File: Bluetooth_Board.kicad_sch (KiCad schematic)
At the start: 67 parts, among them IC1 STM32WB55CGU6, J1 USART1_Headers, J10 Debug_Pins, J12 Power_Selector_Jumper, J13 General_Pin_Header, J14 JST_XH_2.54_Plug, J15 LPUART1_Headers, J16 SPI1_Headers, J19 3V_Selection_Header, J2 SMA PCB END LAUNCH JACK ROUND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, J3 User Button Jumper, J4 Coin Battery Jumper, J5 USB_B_Micro, J6 I2C1_Headers, J7 General_Pin_Header, J8 BOOT0_Jumper, Q1 MOSFET_SI2333DDS-T1-BE3, U3 USBLC6-2SC6, Y4 ABM3B-32.000MHZ-8-R30-B1U-T

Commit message: Update
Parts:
- removed BH1: Battery_Holder_1060TR, Personal_Project:Battery_Holder_1060TR, symbol Personal_Projects:Battery_Holder_1060TR
- removed C12: 0p8 GRM1555C1HR80BA01D, Capacitor_SMD:C_0402_1005Metric_Pad0.74x0.62mm_HandSolder, symbol Device:C
- removed C19: 10n, Capacitor_SMD:C_0805_2012Metric, symbol Device:C
- removed C2, C28, C31, C32: 4u7, Capacitor_SMD:C_0805_2012Metric, symbol Device:C
- removed C20, C21, C22, C27, C29, C30, C33, C34: 100n, Capacitor_SMD:C_0805_2012Metric, symbol Device:C
- removed C24, C25, C35: 1u, Capacitor_SMD:C_0805_2012Metric, symbol Device:C
- removed C36, C9: 1uF, Capacitor_SMD:C_0805_2012Metric, symbol Device:C
- removed C7: 0p3 GRM1555C1HR30WA01D, Capacitor_SMD:C_0402_1005Metric_Pad0.74x0.62mm_HandSolder, symbol Device:C
- removed D1: BZX84C4V3LT1G, Package_TO_SOT_SMD:SOT-23, symbol Diode:BZX84Cxx
- removed D2: BZX84C6V2LT1G, Package_TO_SOT_SMD:SOT-23, symbol Diode:BZX84Cxx
- removed FB1: BLM21PG601SN1D_0805, Capacitor_SMD:C_0805_2012Metric, symbol Device:FerriteBead
- removed FLT1: DLF162500LT-5028A1, Personal_Project:DLF162500LT-5028A1, symbol Personal_Projects:DLF162500LT-5028A1
- removed H1, H2, H3, H4: MountingHole_Pad, MountingHole:MountingHole_3.2mm_M3_Pad, symbol Mechanical:MountingHole_Pad
- removed IC1: STM32WB55CGU6, Personal_Project:STM32WB55CGU6_QFN50P700X700X60-49N-D, symbol Personal_Projects:STM32WB55CGU6
- removed J1: USART1_Headers, Connector_PinHeader_2.54mm:PinHeader_2x03_P2.54mm_Horizontal, symbol Connector_Generic:Conn_02x03_Odd_Even
- removed J10: Debug_Pins, Connector_PinHeader_2.54mm:PinHeader_2x04_P2.54mm_Horizontal, symbol Connector_Generic:Conn_02x04_Odd_Even
- removed J12: Power_Selector_Jumper, Connector_PinHeader_2.54mm:PinHeader_2x03_P2.54mm_Vertical, symbol Connector_Generic:Conn_02x03_Odd_Even
- removed J13, J7: General_Pin_Header, Connector_PinHeader_2.54mm:PinHeader_2x07_P2.54mm_Horizontal, symbol Connector_Generic:Conn_02x07_Odd_Even
- removed J14: JST_XH_2.54_Plug, Personal_Project:Connector_Power2pin_SHDRRA2W80P0X250_1X2_740X1150X610P, symbol Personal_Projects:Connector_Power2pin_JST_XH_2.54_Plug
- removed J15: LPUART1_Headers, Connector_PinHeader_2.54mm:PinHeader_2x03_P2.54mm_Horizontal, symbol Connector_Generic:Conn_02x03_Odd_Even
- removed J16: SPI1_Headers, Connector_PinHeader_2.54mm:PinHeader_2x03_P2.54mm_Horizontal, symbol Connector_Generic:Conn_02x03_Odd_Even
- removed J19: 3V_Selection_Header, Connector_PinHeader_2.54mm:PinHeader_1x03_P2.54mm_Vertical, symbol Connector_Generic:Conn_01x03
- removed J2: SMA PCB END LAUNCH JACK ROUND PO, Personal_Project:SMA Clip Mount Adapter (top), symbol Personal_Projects:SMA PCB END LAUNCH JACK ROUND PO
- removed J3: User Button Jumper, Connector_PinHeader_2.54mm:PinHeader_1x02_P2.54mm_Vertical, symbol Connector_Generic:Conn_01x02
- removed J4: Coin Battery Jumper, Connector_PinHeader_2.54mm:PinHeader_1x03_P2.54mm_Vertical, symbol Connector_Generic:Conn_01x03
- removed J5: USB_B_Micro, Connector_USB:USB_Micro-B_XKB_U254-051T-4BH83-F1S, symbol Connector:USB_B_Micro
- removed J6: I2C1_Headers, Connector_PinHeader_2.54mm:PinHeader_2x03_P2.54mm_Horizontal, symbol Connector_Generic:Conn_02x03_Odd_Even
- removed J8: BOOT0_Jumper, Connector_PinHeader_2.54mm:PinHeader_1x03_P2.54mm_Vertical, symbol Connector:Conn_01x03_Pin
- removed L1: 2n7 LQG15HS2N7S02, Inductor_SMD:L_0402_1005Metric_Pad0.77x0.64mm_HandSolder, symbol Device:L
- removed L4: 10u Murata LQM21FN100M70L, Inductor_SMD:L_0805_2012Metric_Pad1.15x1.40mm_HandSolder, symbol Device:L
- removed L5: 10n Murata LQG15WZ10NJ02D, Inductor_SMD:L_0402_1005Metric_Pad0.77x0.64mm_HandSolder, symbol Device:L
- removed LDO1: LDO_TLV75733PDBVR, Personal_Project:LDO_SOT95P280X145-5N, symbol Personal_Projects:LDO_TLV75733PDBVR
- removed OS2: Oscillator_ECS-327MVATX-3-CN-TR, Personal_Project:Oscillator_ECS327MVATX3CNTR, symbol Personal_Projects:Oscillator_ECS-327MVATX-3-CN-TR
- removed Q1: MOSFET_SI2333DDS-T1-BE3, Personal_Project:MOSFET_ SI2333DDS_SOT_DS-T1-BE3_VIS, symbol Personal_Projects:MOSFET_SI2333DDS-T1-BE3
- removed R1, R10, R11, R12, R13, R14, R3: 33R, Resistor_SMD:R_0805_2012Metric, symbol Device:R
- removed R2: 10R, Resistor_SMD:R_0805_2012Metric, symbol Device:R
- removed R20, R6: 100k, Resistor_SMD:R_0805_2012Metric, symbol Device:R
- removed S2: Switch_WS-SLSU SMT Mini Slide, Personal_Project:Switch_WS-SLSU SMT Mini Slide, symbol Personal_Projects:Switch_WS-SLSU SMT Mini Slide
- removed U2, U6: ~, Personal_Project:Button_KMR231GLFS, symbol Personal_Projects:Button_KMR231GLFS
- removed U3: USBLC6-2SC6, Package_TO_SOT_SMD:SOT-23-6, symbol Power_Protection:USBLC6-2SC6
- removed Y4: ABM3B-32.000MHZ-8-R30-B1U-T, Personal_Project:XTAL_ABM3B-32.000MHZ-10-R30-B1U-T, symbol Personal_Projects:ABM3B-32.000MHZ-10-R30-B1U-T
- removed Z1: Diode_BZX84C6V2-7-F, Personal_Project:Diode_BZX84C6V2_SOT96P240X110-3N, symbol Personal_Projects:Diode_BZX84C6V2-7-F
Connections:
- no-connect marks 10 -> 0
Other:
- added sheet Interfaces (Interfaces.kicad_sch)
- added sheet Power_Management (Power_Management.kicad_sch)
- added sheet STM32WB55CGU6 (STM32WB55CGU6.kicad_sch)
- note removed: "120ohm at 100MHz"
- note removed: "2.4 GHz band antenna"
- note removed: "BOOT0 Switch HIGH enables UART or I2C to allow programminng of the MCU"
- note removed: "Can be used as GPIO"
- note removed: "Chip Select pin on general pin header"
- note removed: "Cloock Output"
- note removed: "Decide onn user button location ---------------"
- note removed: "EP is optional adhesive zone"
- note removed: "Footprint: 0402"
- note removed: "If shutdown capability is not required, connect EN to IN."
- note removed: "Input voltage range: 1.45V to 5.5V"
- note removed: "Load Capacitors are inside the MCU Set RCC_HSECR register"
- note removed: "NRST has internal pull-up resistor -When button not pushed NRST is HIGH -Pushing the button causes current to flow and pulls NRST low"
- note removed: "ON/OFF Switch"
- note removed: "On UFQFPN48 VDDA is connected to VREF+."
- note removed: "Overvoltage protection for the PMOSFET VGS (VGS max is 8V)"
- note removed: "PIN1 NC = Oscillation"
- note removed: "Polarity Protection"
- note removed: "ST-LINK Connections: VCP_TX, SWCLK, SWDIO, VCP_RX, NRST"
- note removed: "STM32MP157FAD1 TFBGA257 Pitch 0.5 2x STM32WB55CGU6 2x STM32WB5MMGH6TR STM32MP135DAF7 TFBGA320 Pitch 0.5 STM32H7S7L8H6H STSPIN958TR STM32H7S3I8T6 LSM6DSV16XTR ISM330BXTR STM32WL55CCU6 STM32WL55JCI6 2x AGVLB.25B.07.0060A Connector: I-PEX MHF® I (U.FL Compatible) GW.52.A153 2.4/5.8/7.1GHZ Hinged RP-SMA (M) Connector TI.96.A113 900-940MHZ Connector: SMA(M) CS5381K-KSZ IC 120DB 192KHZ MULTI-BIT ADC 2x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"
- note removed: "The external capacitor on NRST must be placed as close as possible to the device."
- note removed: "The load capacitances are integrated on chip and can be tuned according to the selected crystal via an internal register. By default, the load capacitances are 8 pF for the NX2016 from NDK used on the boards. RCC clock HSE register (RCC_HSECR) Bits 13:8 HSETUNE[5:0]: HSE capacitor tuning Can be changed by software. Do not change when HSE is on. 0x00: minimum load capacitance 0x3F maximum load cap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"
- note removed: "VDDA feeds ADC and DAC pins, and it needs more filtering"

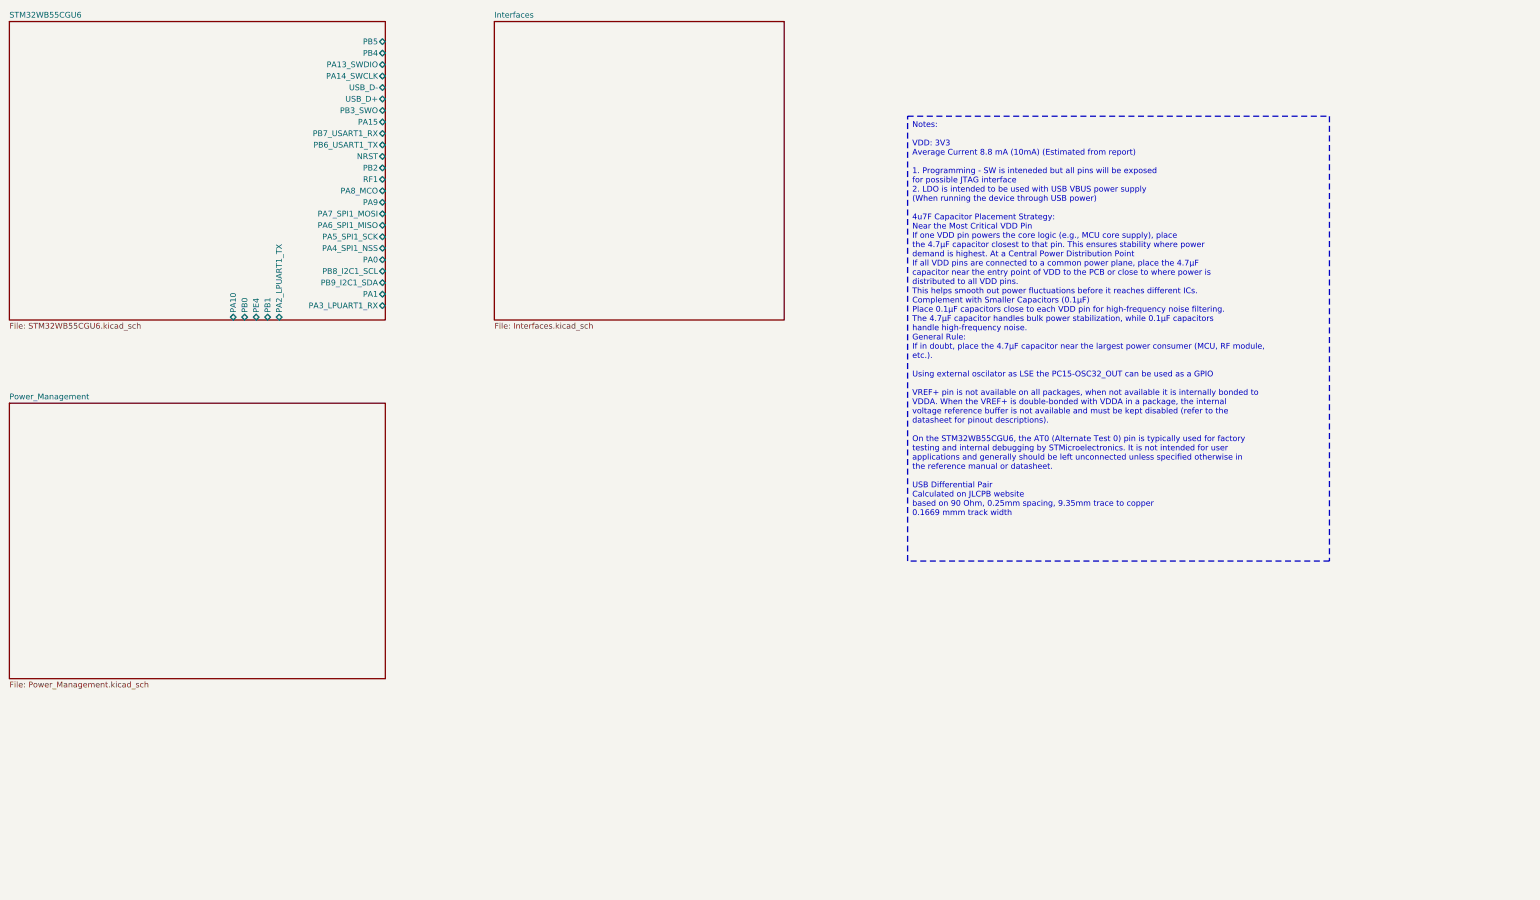
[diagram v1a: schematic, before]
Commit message: Update
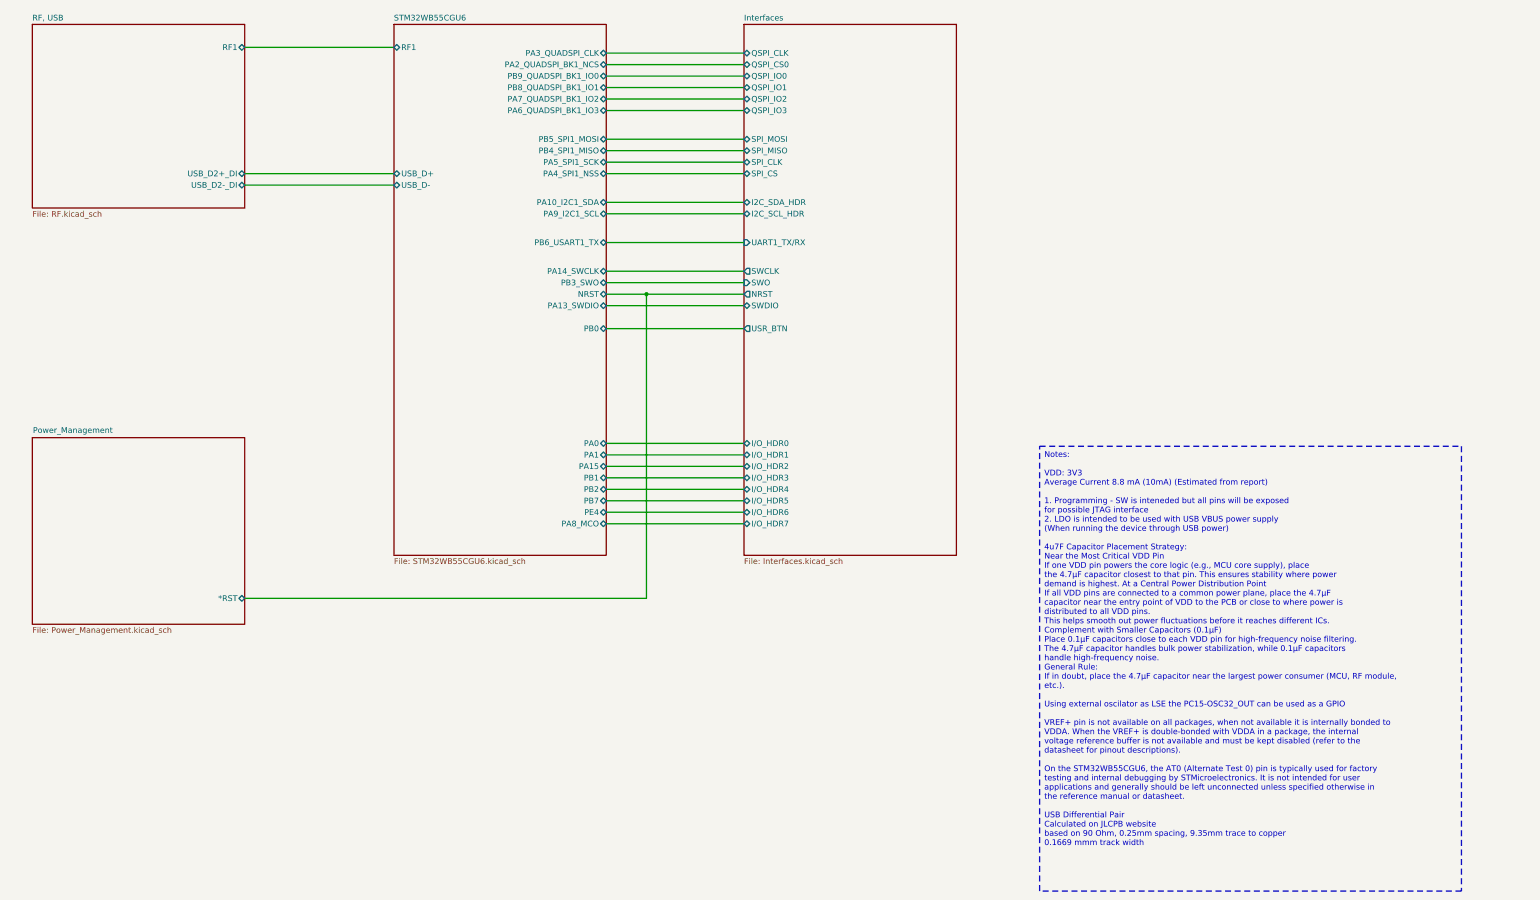
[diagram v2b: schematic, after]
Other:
- added sheet RF, USB (RF.kicad_sch)
- sheet Interfaces ports: added I2C_SCL_HDR, I2C_SDA_HDR, I/O_HDR0, I/O_HDR1, I/O_HDR2, I/O_HDR3, I/O_HDR4, I/O_HDR5, I/O_HDR6, I/O_HDR7, NRST, QSPI_CLK, QSPI_CS0, QSPI_IO0, QSPI_IO1, QSPI_IO2, QSPI_IO3, SPI_CLK, SPI_CS, SPI_MISO, SPI_MOSI, SWCLK, SWDIO, SWO, UART1_TX/RX, USR_BTN; removed none
- sheet Power_Management ports: added *RST; removed none
- sheet STM32WB55CGU6 ports: added PA10_I2C1_SDA, PA2_QUADSPI_BK1_NCS, PA3_QUADSPI_CLK, PA6_QUADSPI_BK1_IO3, PA7_QUADSPI_BK1_IO2, PA9_I2C1_SCL, PB4_SPI1_MISO, PB5_SPI1_MOSI, PB7, PB8_QUADSPI_BK1_IO1, PB9_QUADSPI_BK1_IO0; removed PA10, PA2_LPUART1_TX, PA3_LPUART1_RX, PA6_SPI1_MISO, PA7_SPI1_MOSI, PA9, PB4, PB5, PB7_USART1_RX, PB8_I2C1_SCL, PB9_I2C1_SDA

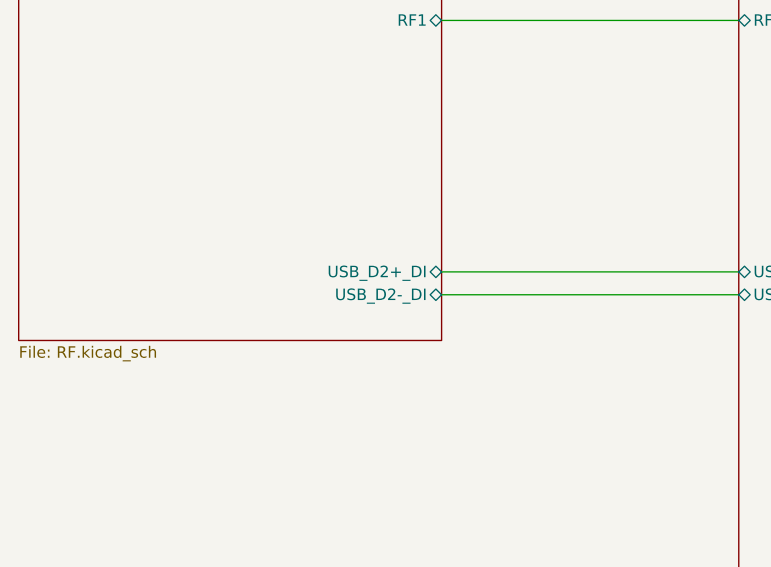
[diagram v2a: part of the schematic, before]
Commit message: Update
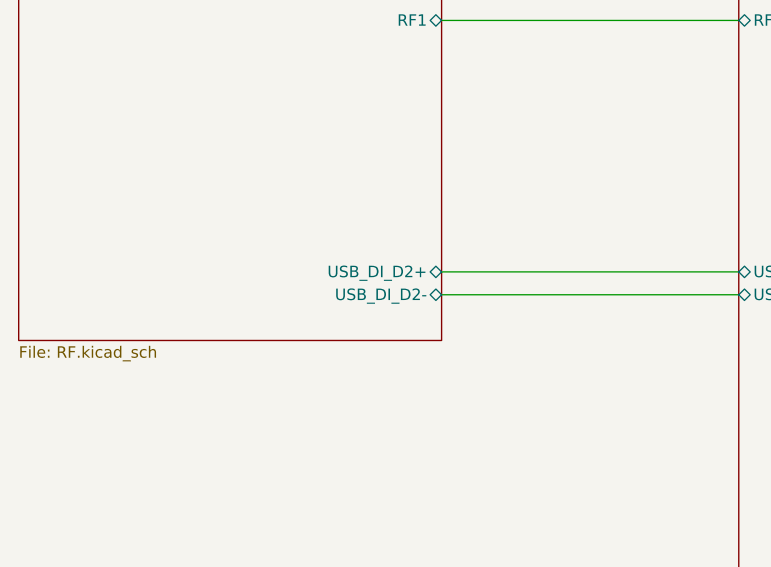
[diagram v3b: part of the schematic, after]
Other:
- sheet RF, USB ports: added USB_DI_D2+, USB_DI_D2-; removed USB_D2+_DI, USB_D2-_DI
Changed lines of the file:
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@@
 			)
 		)
-		(pin "USB_D2+_DI" bidirectional
+		(pin "USB_DI_D2+" bidirectional
 			(at 81.28 60.96 0)
 			(effects
@@
 			)
 		)
-		(pin "USB_D2-_DI" bidirectional
+		(pin "USB_DI_D2-" bidirectional
 			(at 81.28 63.5 0)
 			(effects

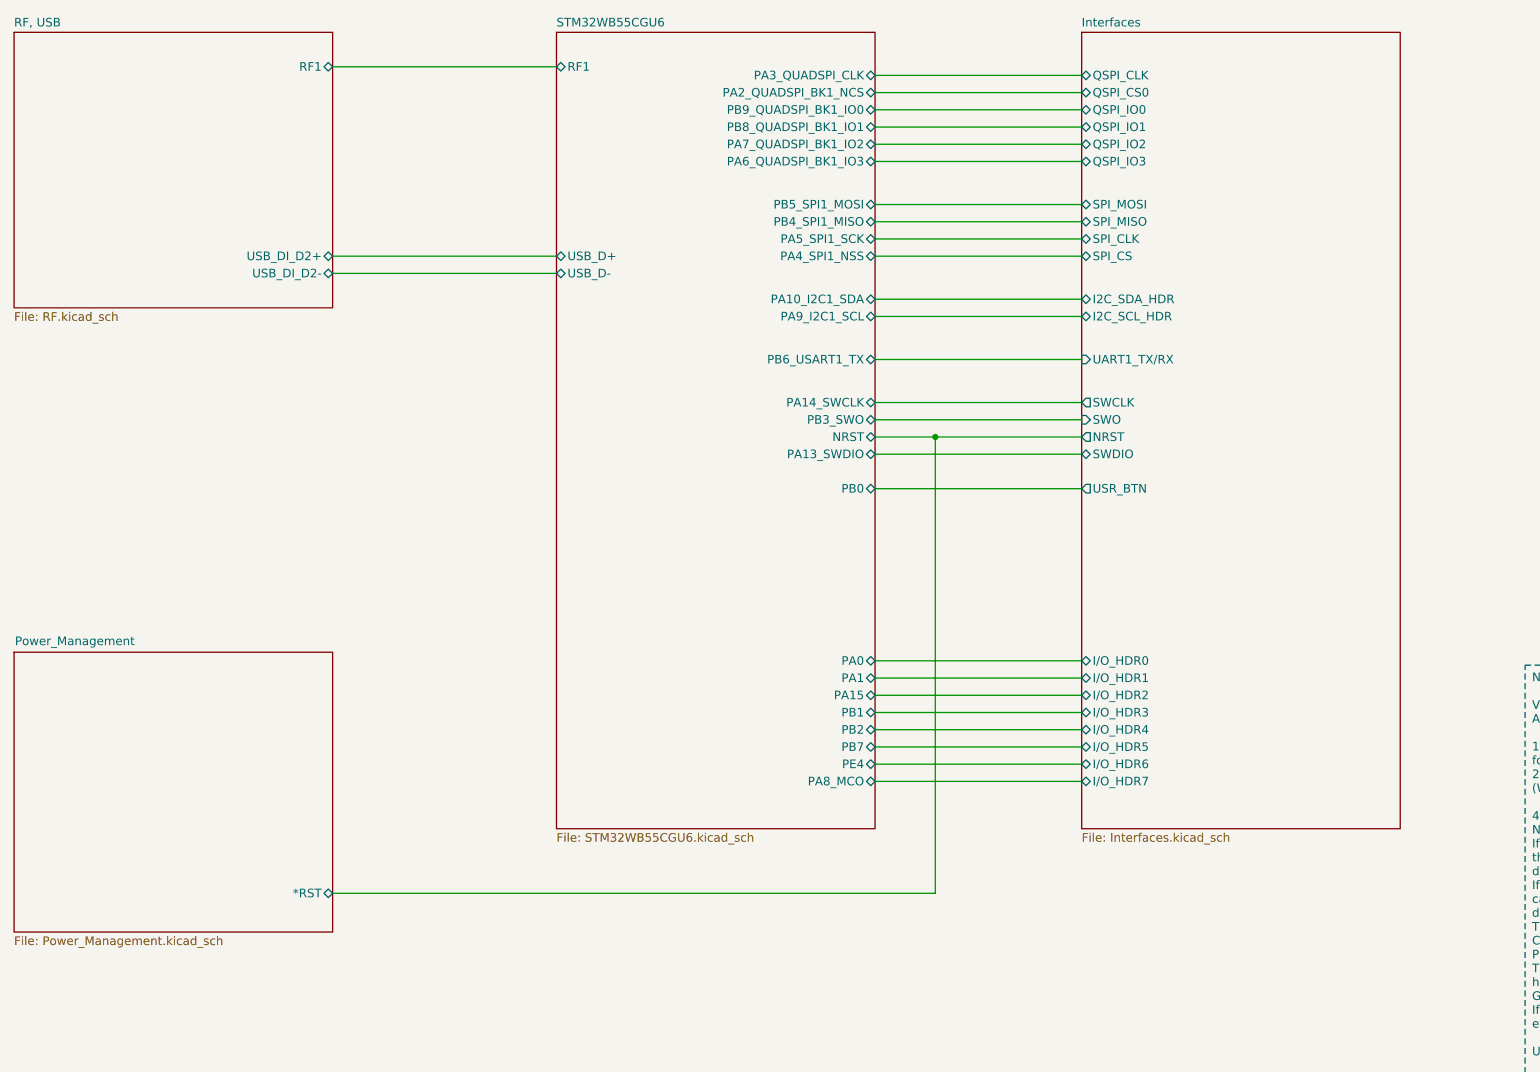
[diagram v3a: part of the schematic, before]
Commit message: Update
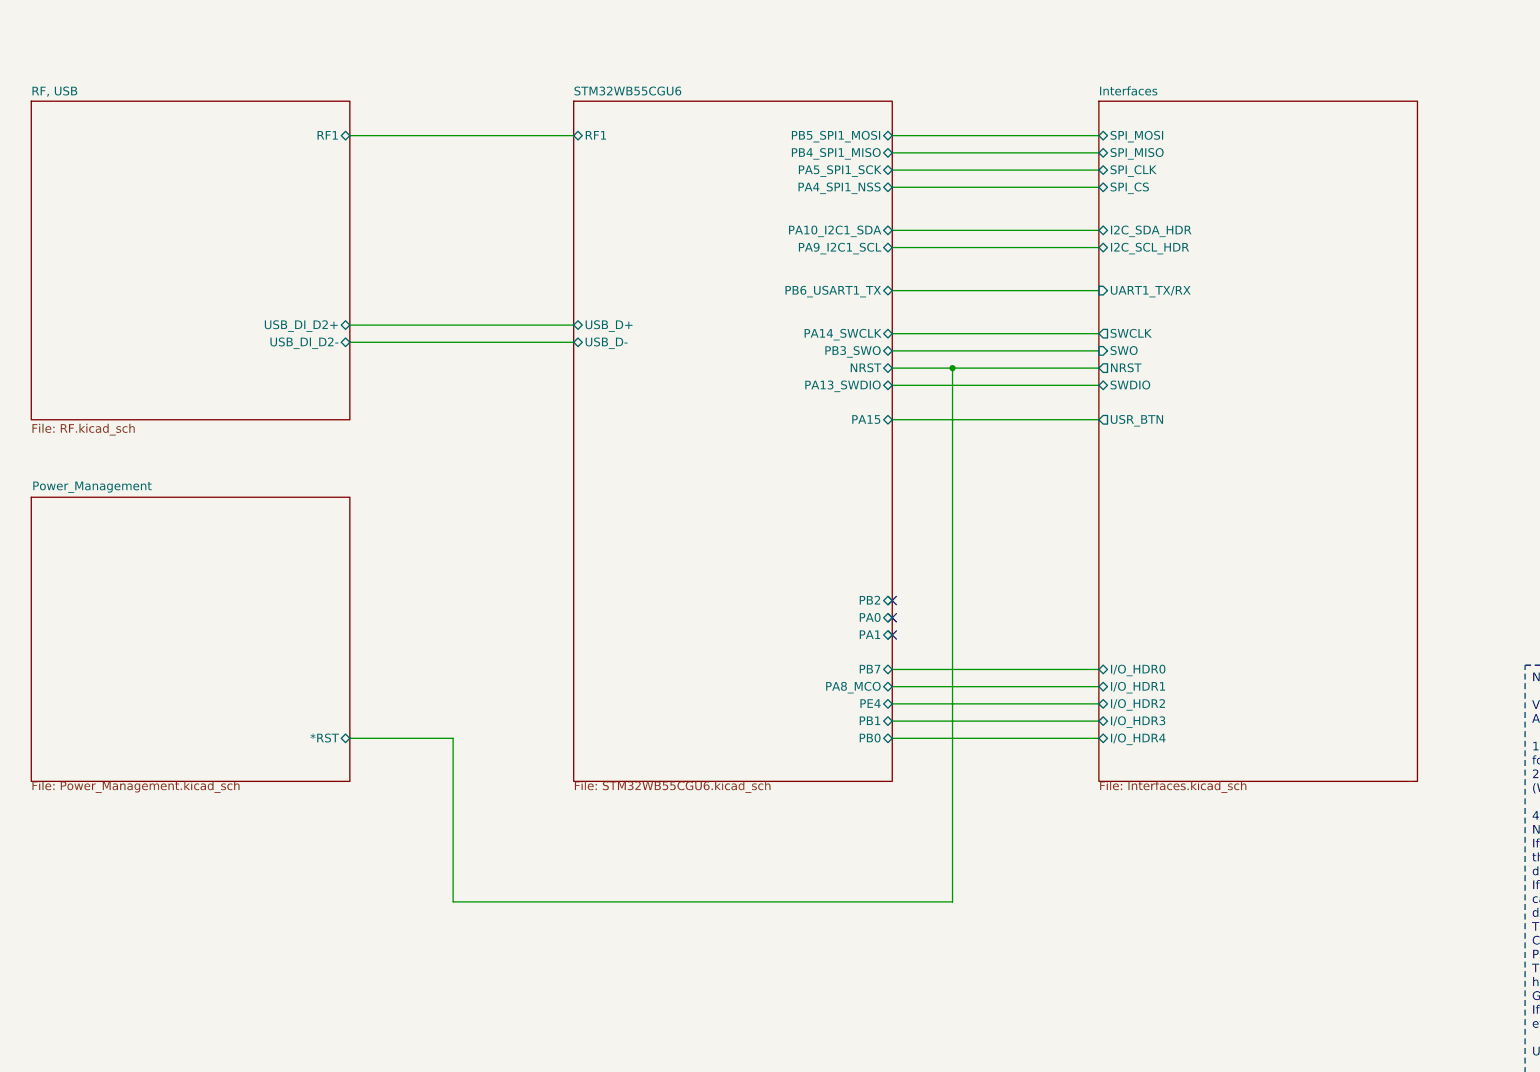
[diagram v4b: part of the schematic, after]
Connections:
- no-connect marks 0 -> 3
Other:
- sheet Interfaces ports: added none; removed I/O_HDR5, I/O_HDR6, I/O_HDR7, QSPI_CLK, QSPI_CS0, QSPI_IO0, QSPI_IO1, QSPI_IO2, QSPI_IO3
- sheet STM32WB55CGU6 ports: added none; removed PA2_QUADSPI_BK1_NCS, PA3_QUADSPI_CLK, PA6_QUADSPI_BK1_IO3, PA7_QUADSPI_BK1_IO2, PB8_QUADSPI_BK1_IO1, PB9_QUADSPI_BK1_IO0
